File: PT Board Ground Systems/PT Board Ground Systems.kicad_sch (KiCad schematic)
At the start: 31 parts, among them J1 OUT CHAN 1, J2 CHAN IN, J3 OUT CHAN 2

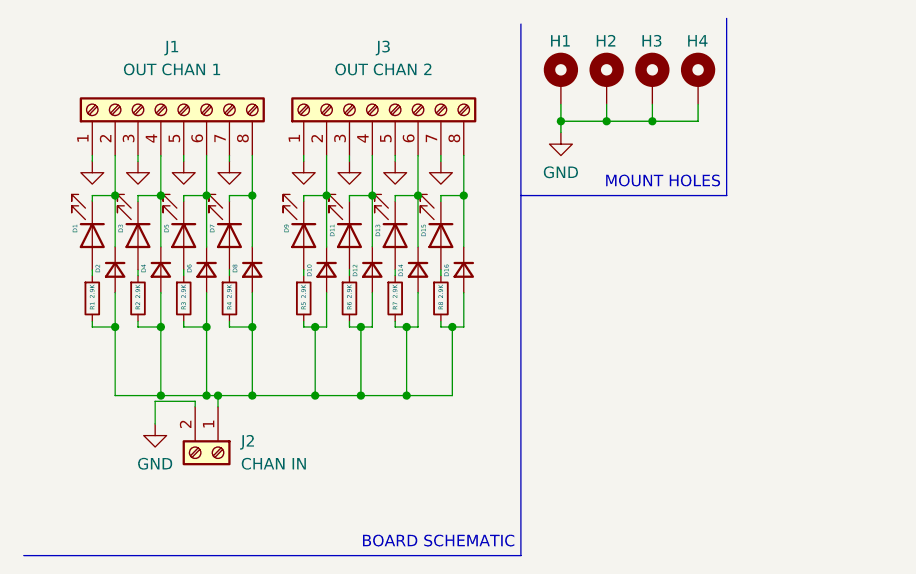
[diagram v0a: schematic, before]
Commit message: AGS Board Work
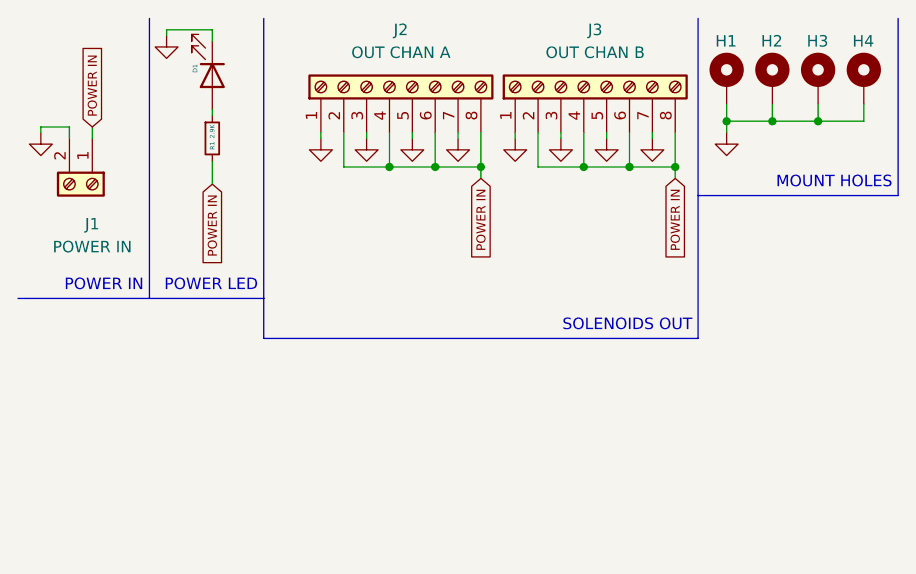
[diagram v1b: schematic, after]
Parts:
- removed D10, D12, D14, D16, D2, D4, D6, D8: D_Small, Diode_SMD:D_SMA, symbol Device:D_Small
- removed D11, D13, D15, D3, D5, D7, D9: LED, LED_SMD:LED_0805_2012Metric, symbol Device:LED
- removed J1: OUT CHAN 1, TerminalBlock_Phoenix:TerminalBlock_Phoenix_MPT-0,5-8-2.54_1x08_P2.54mm_Horizontal, symbol Connector:Screw_Terminal_01x08
- removed J2: CHAN IN, TerminalBlock_Phoenix:TerminalBlock_Phoenix_MPT-0,5-2-2.54_1x02_P2.54mm_Horizontal, symbol Connector:Screw_Terminal_01x02
- removed R2, R3, R4, R5, R6, R7, R8: 2.9K, Resistor_SMD:R_0603_1608Metric, symbol Device:R_Small
- added J1: POWER IN, TerminalBlock_Phoenix:TerminalBlock_Phoenix_MPT-0,5-2-2.54_1x02_P2.54mm_Horizontal, symbol Connector:Screw_Terminal_01x02
- added J2: OUT CHAN A, TerminalBlock_Phoenix:TerminalBlock_Phoenix_MPT-0,5-8-2.54_1x08_P2.54mm_Horizontal, symbol Connector:Screw_Terminal_01x08
- J3: value OUT CHAN 2 -> OUT CHAN B
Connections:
- net GND: now also D1.1 (K), J1.2 (Pin_2), J2.1 (Pin_1), J2.3 (Pin_3), J2.5 (Pin_5), J2.7 (Pin_7)
- net POWER IN: now reaches J3.2 (Pin_2)
- net POWER IN: now also J3.4 (Pin_4), J3.6 (Pin_6), J3.8 (Pin_8), R1.2, J1.1 (Pin_1), J2.2 (Pin_2), J2.4 (Pin_4), J2.6 (Pin_6), J2.8 (Pin_8)
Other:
- note added: "POWER IN"
- note added: "POWER LED"
- note added: "SOLENOIDS OUT"
- note removed: "BOARD SCHEMATIC"
